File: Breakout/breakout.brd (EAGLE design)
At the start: 52.6 x 42.5 mm, 49 parts, among them Q1 16Mhz, U1 TPS63001DRCT, U11 XL

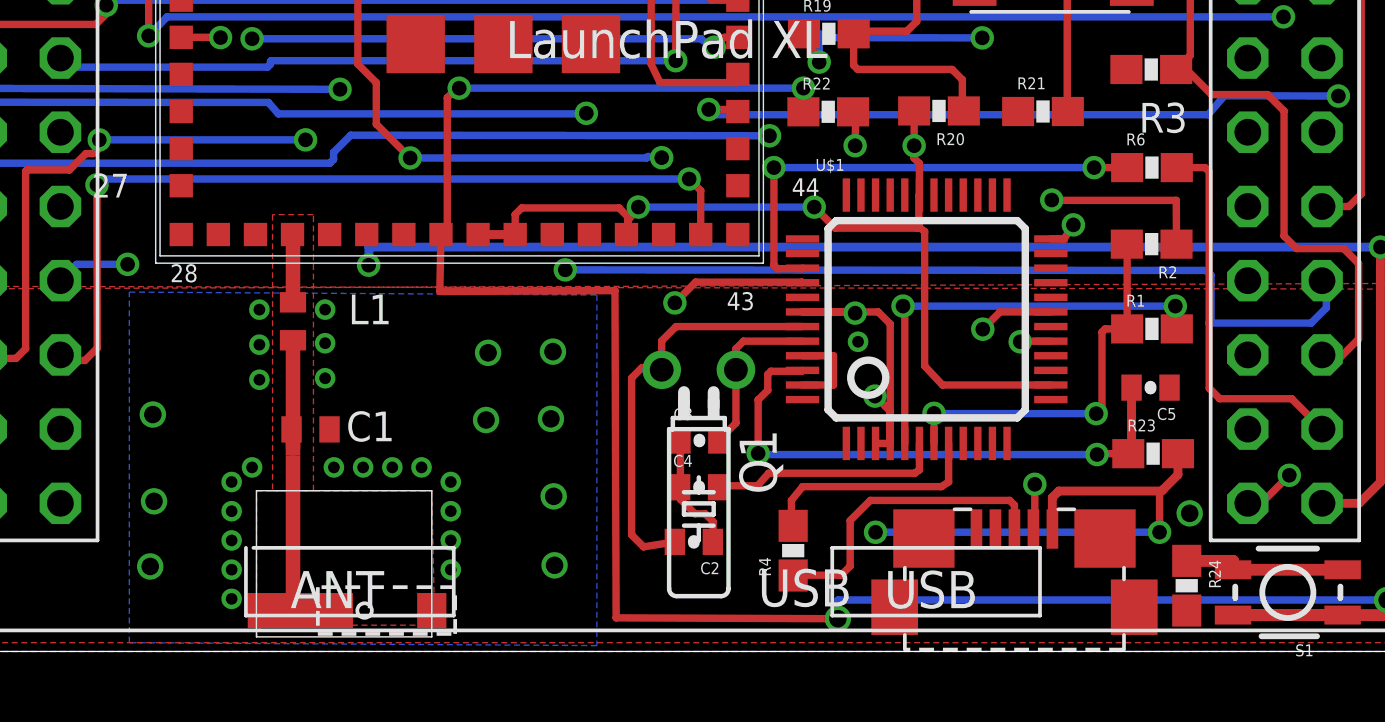
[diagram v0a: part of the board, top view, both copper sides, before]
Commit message: more ground fixed
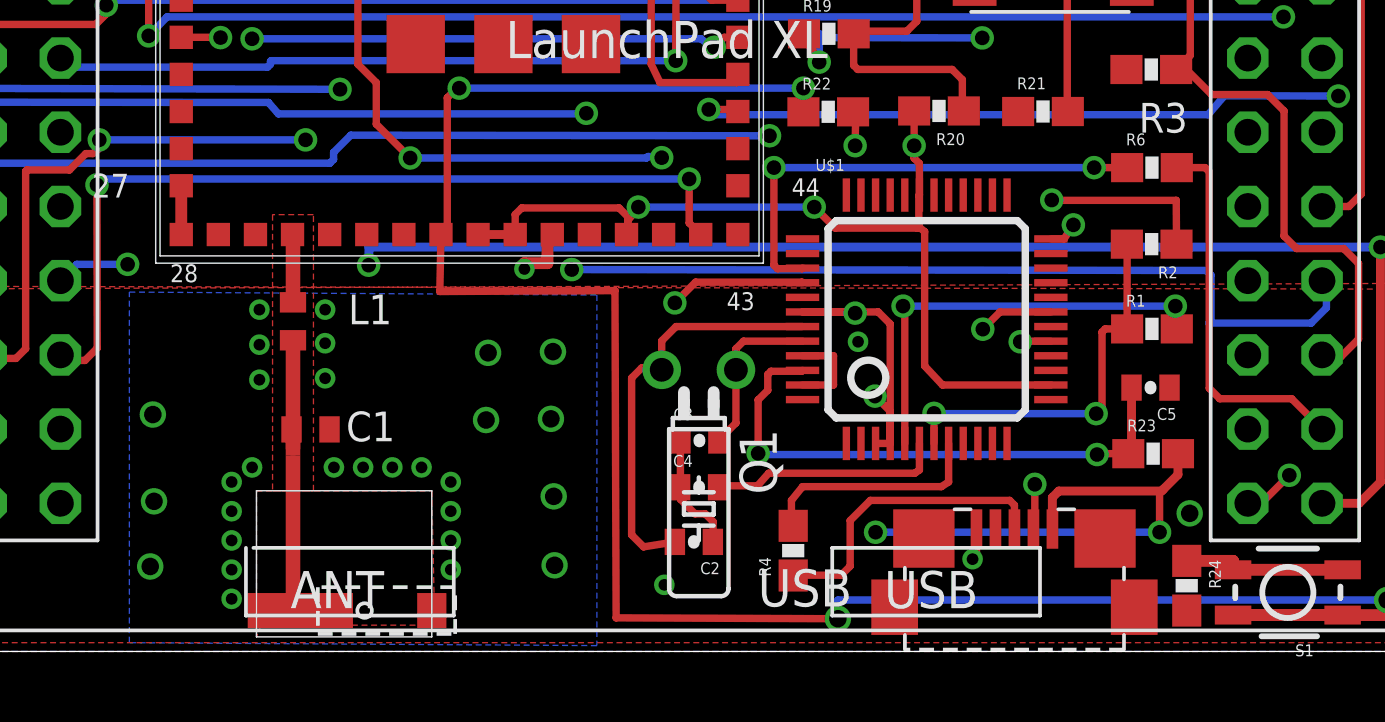
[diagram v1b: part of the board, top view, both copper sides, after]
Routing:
- net GND: track 32.1 -> 36.9 mm, vias 39 -> 42
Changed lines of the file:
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@@
 <wire x1="40.28" y1="4.44" x2="40.28" y2="3.76" width="0.254" layer="1"/>
 <wire x1="40.28" y1="3.76" x2="40.27" y2="3.75" width="0.254" layer="1"/>
-<wire x1="58.39" y1="32.79" x2="61.12" y2="27.93" width="0" layer="19" extent="1-1"/>
-<wire x1="51.0534" y1="37.5586" x2="58.39" y2="32.79" width="0" layer="19" extent="1-1"/>
-<wire x1="48.7334" y1="37.5586" x2="51.0534" y2="37.5586" width="0" layer="19" extent="1-1"/>
-<wire x1="41.586" y1="37.366" x2="48.7334" y2="37.5586" width="0" layer="19" extent="1-1"/>
-<wire x1="38.39" y1="36.5908" x2="41.586" y2="37.366" width="0" layer="19" extent="1-1"/>
-<wire x1="40.7934" y1="31.4986" x2="39.86" y2="31.72" width="0" layer="19" extent="1-1"/>
-<wire x1="35.85" y1="26.54" x2="39.85" y2="30.315" width="0" layer="19" extent="1-1"/>
-<wire x1="36.1" y1="23.79" x2="35.85" y2="26.54" width="0" layer="19" extent="1-1"/>
-<wire x1="33.1" y1="26.79" x2="35.85" y2="26.54" width="0" layer="19" extent="1-1"/>
-<wire x1="33.1" y1="23.79" x2="36.1" y2="23.79" width="0" layer="19" extent="1-1"/>
-<wire x1="36.1" y1="20.79" x2="36.1" y2="23.79" width="0" layer="19" extent="1-1"/>
-<wire x1="33.1" y1="20.79" x2="33.1" y2="23.79" width="0" layer="19" extent="1-1"/>
-<wire x1="30.1" y1="26.79" x2="33.1" y2="26.79" width="0" layer="19" extent="1-1"/>
-<wire x1="30.1" y1="23.79" x2="33.1" y2="23.79" width="0" layer="19" extent="1-1"/>
-<wire x1="30.1" y1="20.79" x2="33.1" y2="20.79" width="0" layer="19" extent="1-1"/>
-<wire x1="34.775" y1="14.27" x2="36.1" y2="20.79" width="0" layer="19" extent="1-1"/>
-<wire x1="34.798" y1="10.2616" x2="34.775" y2="14.27" width="0" layer="19" extent="1-1"/>
-<wire x1="32.578" y1="10.2216" x2="34.798" y2="10.2616" width="0" layer="19" extent="1-1"/>
-<wire x1="34.728" y1="7.9616" x2="34.798" y2="10.2616" width="0" layer="19" extent="1-1"/>
-<wire x1="32.508" y1="7.9216" x2="34.728" y2="7.9616" width="0" layer="19" extent="1-1"/>
-<wire x1="31.3" y1="5.8" x2="32.508" y2="7.9216" width="0" layer="19" extent="1-1"/>
-<wire x1="31.3" y1="4.8" x2="31.3" y2="5.8" width="0" layer="19" extent="1-1"/>
-<wire x1="31.3" y1="3.8" x2="31.3" y2="4.8" width="0" layer="19" extent="1-1"/>
-<wire x1="31.3" y1="2.8" x2="31.3" y2="3.8" width="0" layer="19" extent="1-1"/>
-<wire x1="30.3" y1="6.3" x2="31.3" y2="5.8" width="0" layer="19" extent="1-1"/>
-<wire x1="29.3" y1="6.3" x2="30.3" y2="6.3" width="0" layer="19" extent="1-1"/>
-<wire x1="28.3" y1="6.3" x2="29.3" y2="6.3" width="0" layer="19" extent="1-1"/>
-<wire x1="27.3" y1="6.3" x2="28.3" y2="6.3" width="0" layer="19" extent="1-1"/>
-<wire x1="27.15" y1="7.6" x2="27.3" y2="6.3" width="0" layer="19" extent="1-1"/>
-<wire x1="30.65" y1="1.4" x2="31.3" y2="2.8" width="0" layer="19" extent="1-1"/>
-<wire x1="27" y1="9.35" x2="27.15" y2="7.6" width="0" layer="19" extent="1-1"/>
-<wire x1="27" y1="10.55" x2="27" y2="9.35" width="0" layer="19" extent="1-1"/>
-<wire x1="27" y1="11.7" x2="27" y2="10.55" width="0" layer="19" extent="1-1"/>
-<wire x1="24.75" y1="10.5" x2="27" y2="10.55" width="0" layer="19" extent="1-1"/>
-<wire x1="24.75" y1="11.7" x2="24.75" y2="10.5" width="0" layer="19" extent="1-1"/>
-<wire x1="24.75" y1="9.3" x2="24.75" y2="10.5" width="0" layer="19" extent="1-1"/>
-<wire x1="27.155" y1="14.27" x2="27" y2="11.7" width="0" layer="19" extent="1-1"/>
-<wire x1="24.615" y1="14.27" x2="27.155" y2="14.27" width="0" layer="19" extent="1-1"/>
-<wire x1="22.075" y1="14.27" x2="24.615" y2="14.27" width="0" layer="19" extent="1-1"/>
-<wire x1="22.075" y1="15.94" x2="22.075" y2="14.27" width="0" layer="19" extent="1-1"/>
-<wire x1="34.8234" y1="5.3086" x2="34.728" y2="7.9616" width="0" layer="19" extent="1-1"/>
-<wire x1="34.8534" y1="2.9486" x2="34.8234" y2="5.3086" width="0" layer="19" extent="1-1"/>
-<wire x1="24.5" y1="6.3" x2="27.3" y2="6.3" width="0" layer="19" extent="1-1"/>
-<wire x1="23.8" y1="5.8" x2="24.5" y2="6.3" width="0" layer="19" extent="1-1"/>
-<wire x1="23.8" y1="4.8" x2="23.8" y2="5.8" width="0" layer="19" extent="1-1"/>
-<wire x1="23.8" y1="3.8" x2="23.8" y2="4.8" width="0" layer="19" extent="1-1"/>
-<wire x1="23.8" y1="2.8" x2="23.8" y2="3.8" width="0" layer="19" extent="1-1"/>
-<wire x1="23.8" y1="1.8" x2="23.8" y2="2.8" width="0" layer="19" extent="1-1"/>
-<wire x1="24.5" y1="1.4" x2="23.8" y2="1.8" width="0" layer="19" extent="1-1"/>
-<wire x1="21.1434" y1="5.1386" x2="23.8" y2="4.8" width="0" layer="19" extent="1-1"/>
-<wire x1="21.0134" y1="2.9086" x2="21.1434" y2="5.1386" width="0" layer="19" extent="1-1"/>
-<wire x1="21.1034" y1="8.1086" x2="21.1434" y2="5.1386" width="0" layer="19" extent="1-1"/>
-<wire x1="39.15" y1="5.62" x2="34.8234" y2="5.3086" width="0" layer="19" extent="1-1"/>
-<wire x1="43.34" y1="9.12" x2="39.16" y2="7.22" width="0" layer="19" extent="1-1"/>
-<wire x1="45.24" y1="10.6" x2="44.4" y2="10.12" width="0" layer="19" extent="1-1"/>
-<wire x1="41.125" y1="14.27" x2="43.34" y2="10.12" width="0" layer="19" extent="1-1"/>
-<wire x1="48.84" y1="7.12" x2="44.4" y2="9.12" width="0" layer="19" extent="1-1"/>
-<wire x1="49.2928" y1="4.19" x2="48.84" y2="7.12" width="0" layer="19" extent="1-1"/>
-<wire x1="45.84" y1="15.62" x2="41.125" y2="14.27" width="0" layer="19" extent="1-1"/>
+<wire x1="22.075" y1="15.94" x2="22.075" y2="14.27" width="0.4064" layer="1"/>
+<via x="33.82" y="13.09" extent="1-16" drill="0.4"/>
+<wire x1="34.775" y1="14.27" x2="34.61" y2="14.27" width="0.4064" layer="1"/>
+<wire x1="34.61" y1="14.27" x2="34.61" y2="13.29" width="0.4064" layer="1"/>
+<wire x1="34.61" y1="13.29" x2="33.82" y2="13.29" width="0.4064" layer="1"/>
+<wire x1="33.82" y1="13.29" x2="33.82" y2="13.09" width="0.4064" layer="1"/>
+<via x="38.61" y="2.28" extent="1-16" drill="0.4"/>
+<via x="49.16" y="3.16" extent="1-16" drill="0.4"/>
 <wire x1="50.34" y1="15.62" x2="45.84" y2="15.62" width="0" layer="19" extent="1-1"/>
-<wire x1="50.72" y1="18.48" x2="50.34" y2="15.62" width="0" layer="19" extent="1-1"/>
-<wire x1="54.426" y1="19.918" x2="50.72" y2="18.48" width="0" layer="19" extent="1-1"/>
-<wire x1="49.23" y1="22.37" x2="50.72" y2="18.48" width="0" layer="19" extent="1-1"/>
-<wire x1="51.84" y1="11.12" x2="50.34" y2="15.62" width="0" layer="19" extent="1-1"/>
-<wire x1="55.9" y1="9.03" x2="51.84" y2="11.12" width="0" layer="19" extent="1-1"/>
-<wire x1="56.5912" y1="4.7264" x2="55.9" y2="9.03" width="0" layer="19" extent="1-1"/>
-<wire x1="56.49" y1="1.4" x2="56.5912" y2="4.7264" width="0" layer="19" extent="1-1"/>
-<wire x1="43.608" y1="22.9916" x2="49.23" y2="22.37" width="0" layer="19" extent="1-1"/>
-<wire x1="27.32" y1="35.09" x2="30.1" y2="26.79" width="0" layer="19" extent="1-1"/>
-<wire x1="23.5" y1="33.54" x2="27.32" y2="35.09" width="0" layer="19" extent="1-16"/>
 <wire x1="22.07" y1="30.315" x2="23.5" y2="33.54" width="0" layer="19" extent="1-16"/>
-<wire x1="21.84" y1="37.19" x2="23.5" y2="33.54" width="0" layer="19" extent="1-16"/>
-<wire x1="21.898" y1="38.5116" x2="21.87" y2="39.77" width="0" layer="19" extent="1-1"/>
-<wire x1="18.118" y1="39.8316" x2="21.87" y2="39.77" width="0" layer="19" extent="1-1"/>
-<wire x1="17.81" y1="34.2" x2="21.84" y2="37.19" width="0" layer="19" extent="1-1"/>
-<wire x1="13.248" y1="34.8016" x2="17.81" y2="34.2" width="0" layer="19" extent="1-1"/>
-<wire x1="17.94" y1="25.39" x2="22.07" y2="30.315" width="0" layer="19" extent="1-1"/>
+<wire x1="49.2928" y1="4.19" x2="49.2928" y2="3.2928" width="0.254" layer="1"/>
+<wire x1="49.2928" y1="3.2928" x2="49.16" y2="3.16" width="0.254" layer="1"/>
 </signal>
 <signal name="N$1">
@@
 <via x="34.85" y="31.12" extent="1-16" drill="0.5"/>
 <wire x1="34.85" y1="31.12" x2="34.86" y2="13.4" width="0.254" layer="15"/>
-<wire x1="34.86" y1="13.4" x2="35.22" y2="13.06" width="0.254" layer="15"/>
-<via x="35.22" y="13.06" extent="1-16" drill="0.5"/>
-<wire x1="35.22" y1="13.06" x2="57.16" y2="13.04" width="0.254" layer="16"/>
+<wire x1="34.86" y1="13.4" x2="35.44" y2="13.07" width="0.254" layer="15"/>
+<via x="35.44" y="13.07" extent="1-16" drill="0.5"/>
+<wire x1="35.44" y1="13.07" x2="57.16" y2="13.04" width="0.254" layer="16"/>
 <wire x1="57.16" y1="13.04" x2="57.32" y2="12.88" width="0.254" layer="16"/>
 <wire x1="57.32" y1="12.88" x2="57.32" y2="11.32" width="0.254" layer="16"/>
@@
 <contactref element="CC3200MOD" pad="P42"/>
 <contactref element="U11" pad="GPIO_30"/>
-<wire x1="39.855" y1="14.27" x2="39.855" y2="15.775" width="0.254" layer="1"/>
-<wire x1="39.855" y1="15.775" x2="39.46" y2="16.17" width="0.254" layer="1"/>
 <via x="39.46" y="16.17" extent="1-16" drill="0.5"/>
 <wire x1="39.46" y1="16.17" x2="19.23" y2="16.17" width="0.254" layer="16"/>
@@
 <wire x1="18.78" y1="9.96" x2="18.13" y2="9.96" width="0.254" layer="1"/>
 <wire x1="18.13" y1="9.96" x2="17.94" y2="10.15" width="0.254" layer="1"/>
+<wire x1="39.46" y1="16.17" x2="39.46" y2="14.665" width="0.254" layer="1"/>
+<wire x1="39.46" y1="14.665" x2="39.855" y2="14.27" width="0.254" layer="1"/>
 </signal>
 <signal name="N$15">
